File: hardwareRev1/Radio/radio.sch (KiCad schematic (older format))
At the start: 38 parts

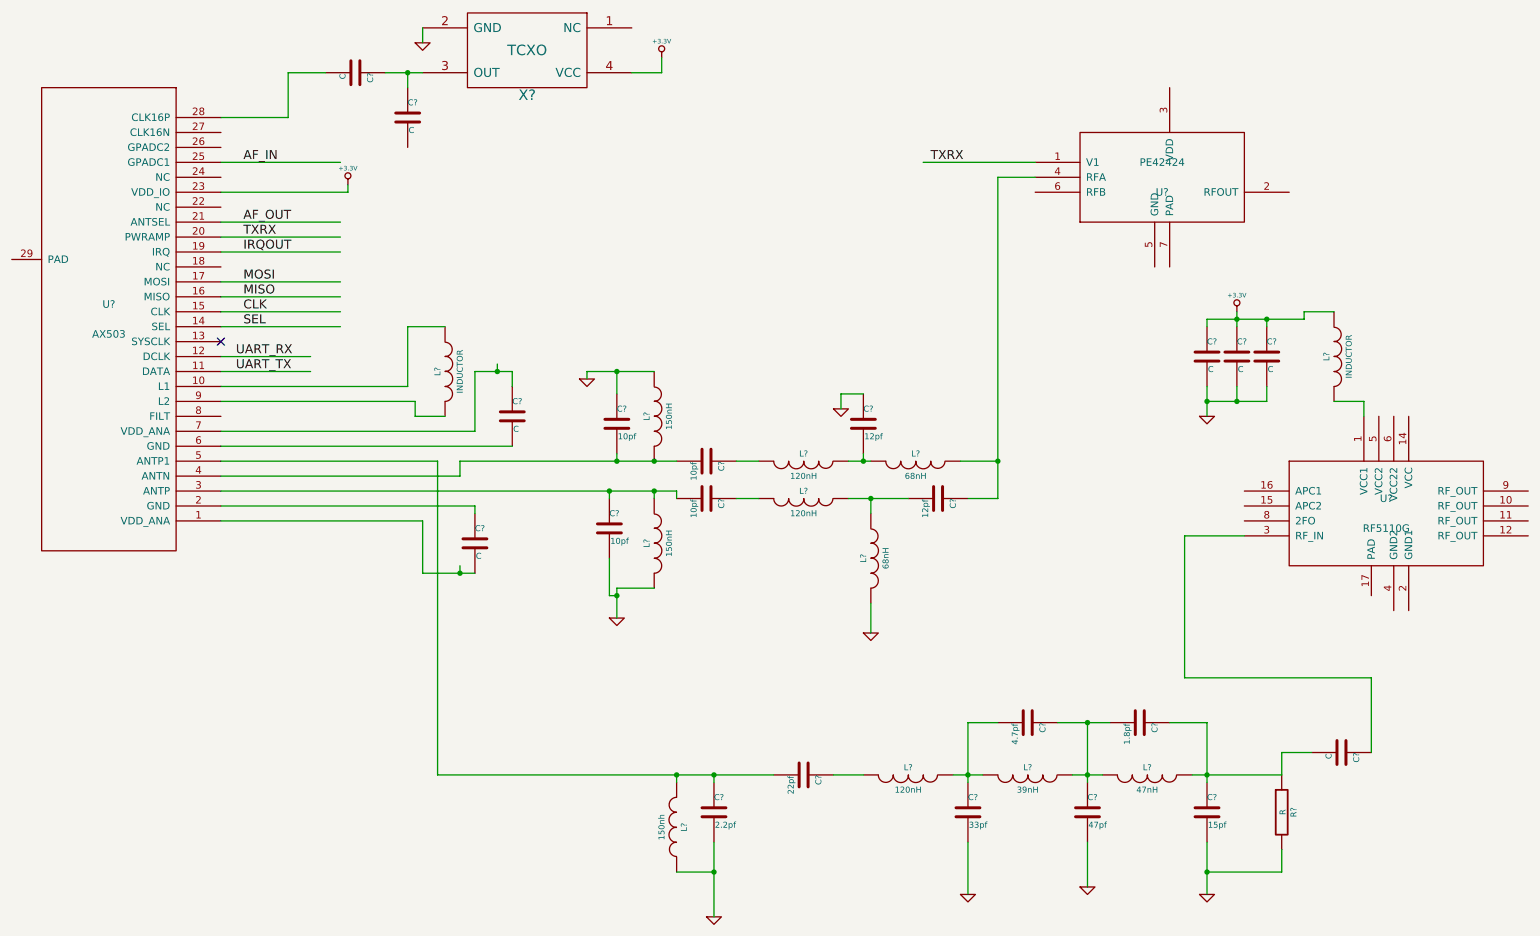
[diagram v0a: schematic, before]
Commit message: finaly back on track
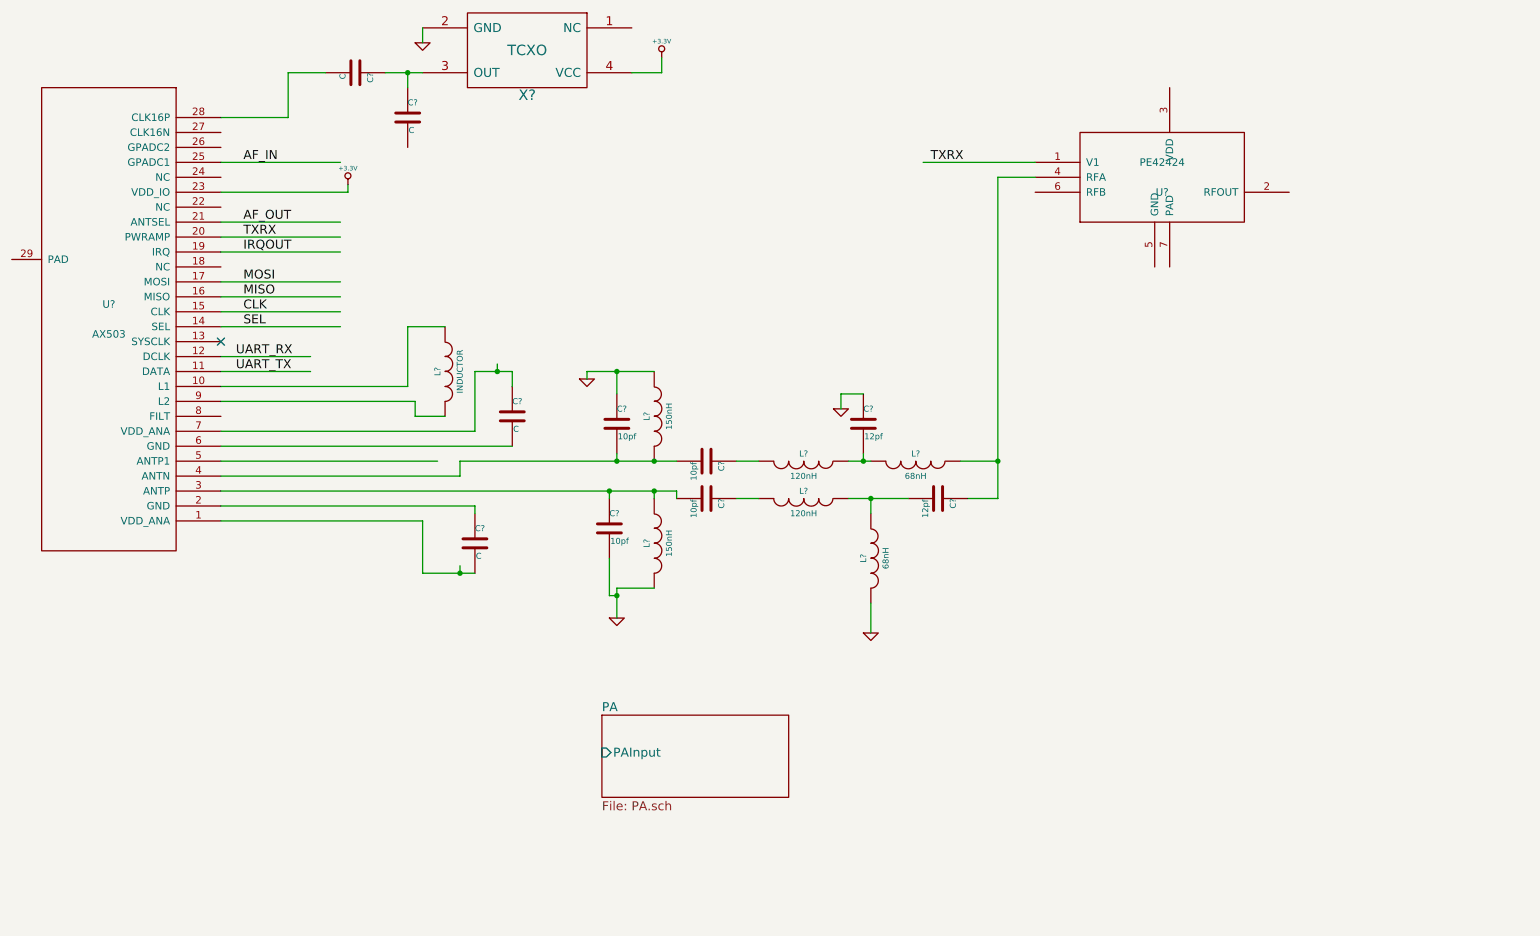
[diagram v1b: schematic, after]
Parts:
- removed C?: 2.2pf, symbol C
- removed C?: 22pf, symbol C
- removed C?: 33pf, symbol C
- removed C?: 47pf, symbol C
- removed C?: 15pf, symbol C
- removed C?: 4.7pf, symbol C
- removed C?: 1.8pf, symbol C
- removed C? (x4): C, symbol C
- removed L?: 150nh, symbol INDUCTOR
- removed L?: 120nH, symbol INDUCTOR
- removed L?: 39nH, symbol INDUCTOR
- removed L?: 47nH, symbol INDUCTOR
- removed L?: INDUCTOR, symbol INDUCTOR
- removed R?: R, symbol R
- removed U?: RF5110G, MODULE, symbol RF5110G
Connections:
- wire segments 107 -> 68
